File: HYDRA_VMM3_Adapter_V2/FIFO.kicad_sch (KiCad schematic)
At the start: 18 parts, among them U2 5PB1213NTGK8, U4 5PB1213NTGK8

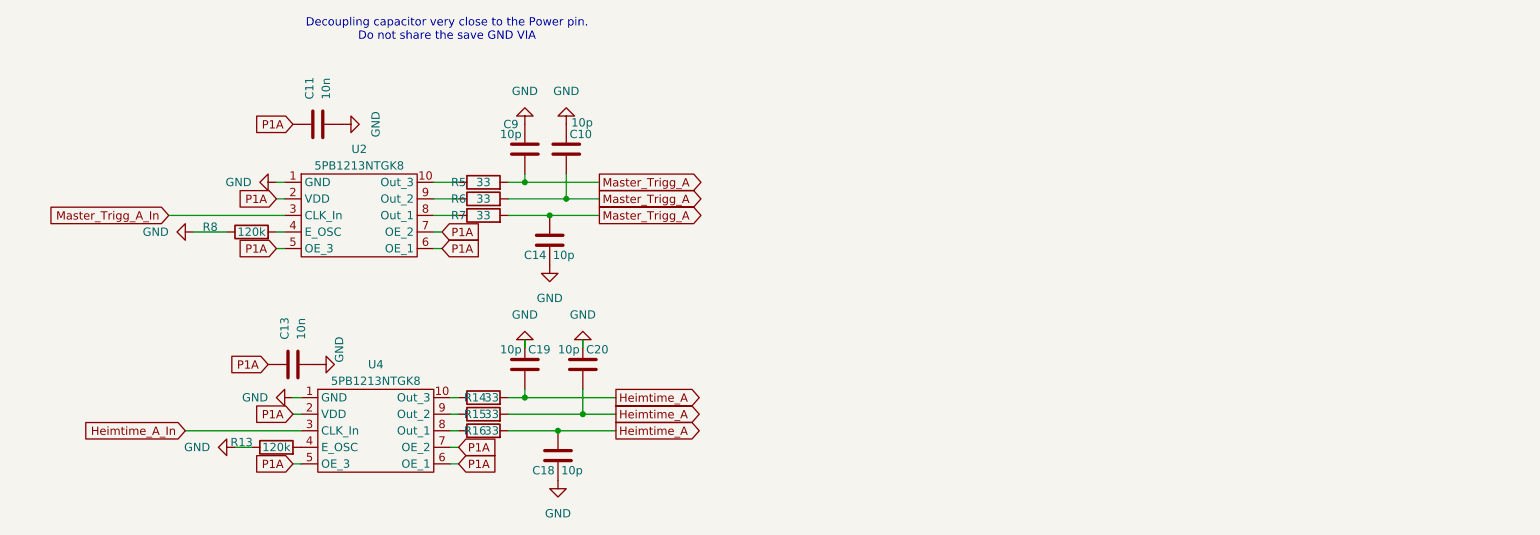
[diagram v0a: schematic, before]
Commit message: .
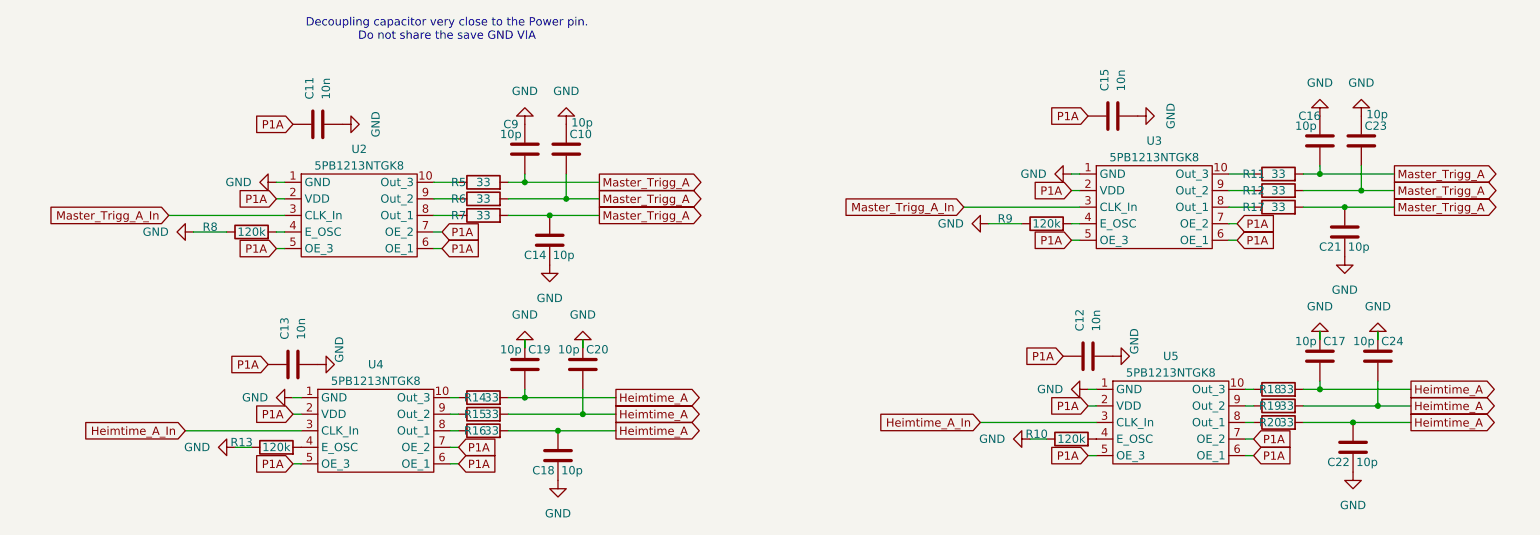
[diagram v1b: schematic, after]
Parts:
- added C12, C15: 10n, Capacitor_SMD:C_0201_0603Metric, symbol Device:C
- added C16, C17, C21, C22, C23, C24: 10p, Capacitor_SMD:C_0201_0603Metric, symbol Device:C
- added R10, R9: 120k, Resistor_SMD:R_0201_0603Metric, symbol Device:R
- added R11, R12, R17, R18, R19, R20: 33, Resistor_SMD:R_0201_0603Metric, symbol Device:R
- added U3, U5: 5PB1213NTGK8, PCI-E_SMD:5PB1213NTGK8, symbol HYDRA_Symbol:5PB1213NTGK8
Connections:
- net GND: now also C12.2, C15.2, C16.1, C17.1, C21.1, C22.1, C23.1, C24.1, R10.1, R9.1, U3.1 (GND), U5.1 (GND)
- net Heimtime_A: now also C17.2, C22.2, C24.2, R18.2, R19.2, R20.2
- net Heimtime_A_In: now also U5.3 (CLK_In)
- net Master_Trigg_A: now also C16.2, C21.2, C23.2, R11.2, R12.2, R17.2
- net Master_Trigg_A_In: now also U3.3 (CLK_In)
- net P1A: now also C12.1, C15.1, U3.2 (VDD), U3.5 (OE_3), U3.6 (OE_1), U3.7 (OE_2), U5.2 (VDD), U5.5 (OE_3), U5.6 (OE_1), U5.7 (OE_2)
- new net: R18.1, U5.10 (Out_3)
- new net: R10.2, U5.4 (E_OSC)
- new net: R20.1, U5.8 (Out_1)
- new net: R19.1, U5.9 (Out_2)
- new net: R9.2, U3.4 (E_OSC)
- new net: R12.1, U3.9 (Out_2)
- new net: R11.1, U3.10 (Out_3)
- new net: R17.1, U3.8 (Out_1)
